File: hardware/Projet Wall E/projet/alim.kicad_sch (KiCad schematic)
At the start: 54 parts, among them J201 USB_C_Receptacle_USB2.0_16P, J202 Conn_01x02, Q201 2SK3019, Q202 MMDT5401, Q203 DMP3099L, U201 AP2112K-3.3, U202 BQ27220YZFR, U203 USBLC6-2SC6, U204 BQ25896RTW

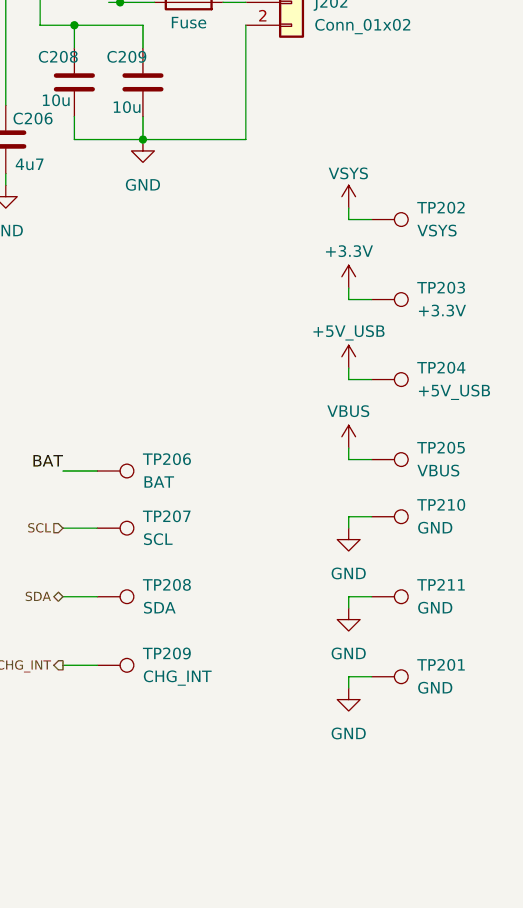
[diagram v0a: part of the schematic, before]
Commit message: PCB : placement final avant routage
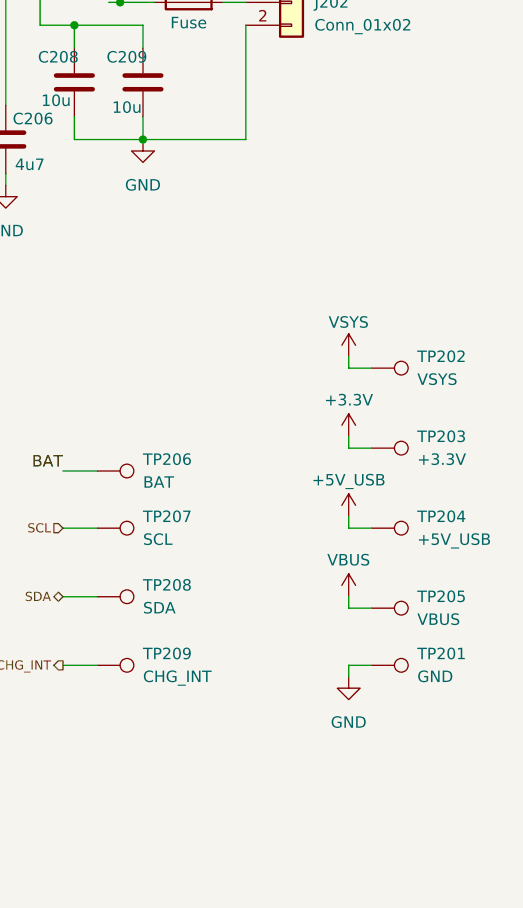
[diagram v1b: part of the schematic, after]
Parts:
- removed TP210, TP211: GND, TestPoint:TestPoint_Pad_D1.5mm, symbol Connector:TestPoint
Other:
- moved on the sheet: TP201, TP202, TP203, TP204, TP205

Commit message: Fichiers de fabrication : Gerbers, perçage, CPL et BOM
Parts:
- TP201, TP202, TP203, TP204, TP205, TP206, TP207, TP208, TP209: now left out of the parts list
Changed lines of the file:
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@@
 		(body_style 1)
 		(exclude_from_sim no)
-		(in_bom yes)
+		(in_bom no)
 		(on_board yes)
 		(in_pos_files yes)
@@
 		(body_style 1)
 		(exclude_from_sim no)
-		(in_bom yes)
+		(in_bom no)
 		(on_board yes)
 		(in_pos_files yes)
@@
 		(body_style 1)
 		(exclude_from_sim no)
-		(in_bom yes)
+		(in_bom no)
 		(on_board yes)
 		(in_pos_files yes)
@@
 		(body_style 1)
 		(exclude_from_sim no)
-		(in_bom yes)
+		(in_bom no)
 		(on_board yes)
 		(in_pos_files yes)
@@
 		(body_style 1)
 		(exclude_from_sim no)
-		(in_bom yes)
+		(in_bom no)
 		(on_board yes)
 		(in_pos_files yes)
@@
 		(body_style 1)
 		(exclude_from_sim no)
-		(in_bom yes)
+		(in_bom no)
 		(on_board yes)
 		(in_pos_files yes)
@@
 		(body_style 1)
 		(exclude_from_sim no)
-		(in_bom yes)
+		(in_bom no)
 		(on_board yes)
 		(in_pos_files yes)
@@
 		(body_style 1)
 		(exclude_from_sim no)
-		(in_bom yes)
+		(in_bom no)
 		(on_board yes)
 		(in_pos_files yes)
@@
 		(body_style 1)
 		(exclude_from_sim no)
-		(in_bom yes)
+		(in_bom no)
 		(on_board yes)
 		(in_pos_files yes)
